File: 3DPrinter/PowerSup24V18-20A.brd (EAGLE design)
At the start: 115 x 161.7 mm, 87 parts, among them IC1 POWER-TNY264PN, T1 TRANS-1/1EFD25-10, T2 _TRANSFORMERS_GDT_20X6.5, T3 TRANS-1/1ETD39, U1 SG3525AN, X1 CON-7.62-02P, X2 CON-7.62-02P

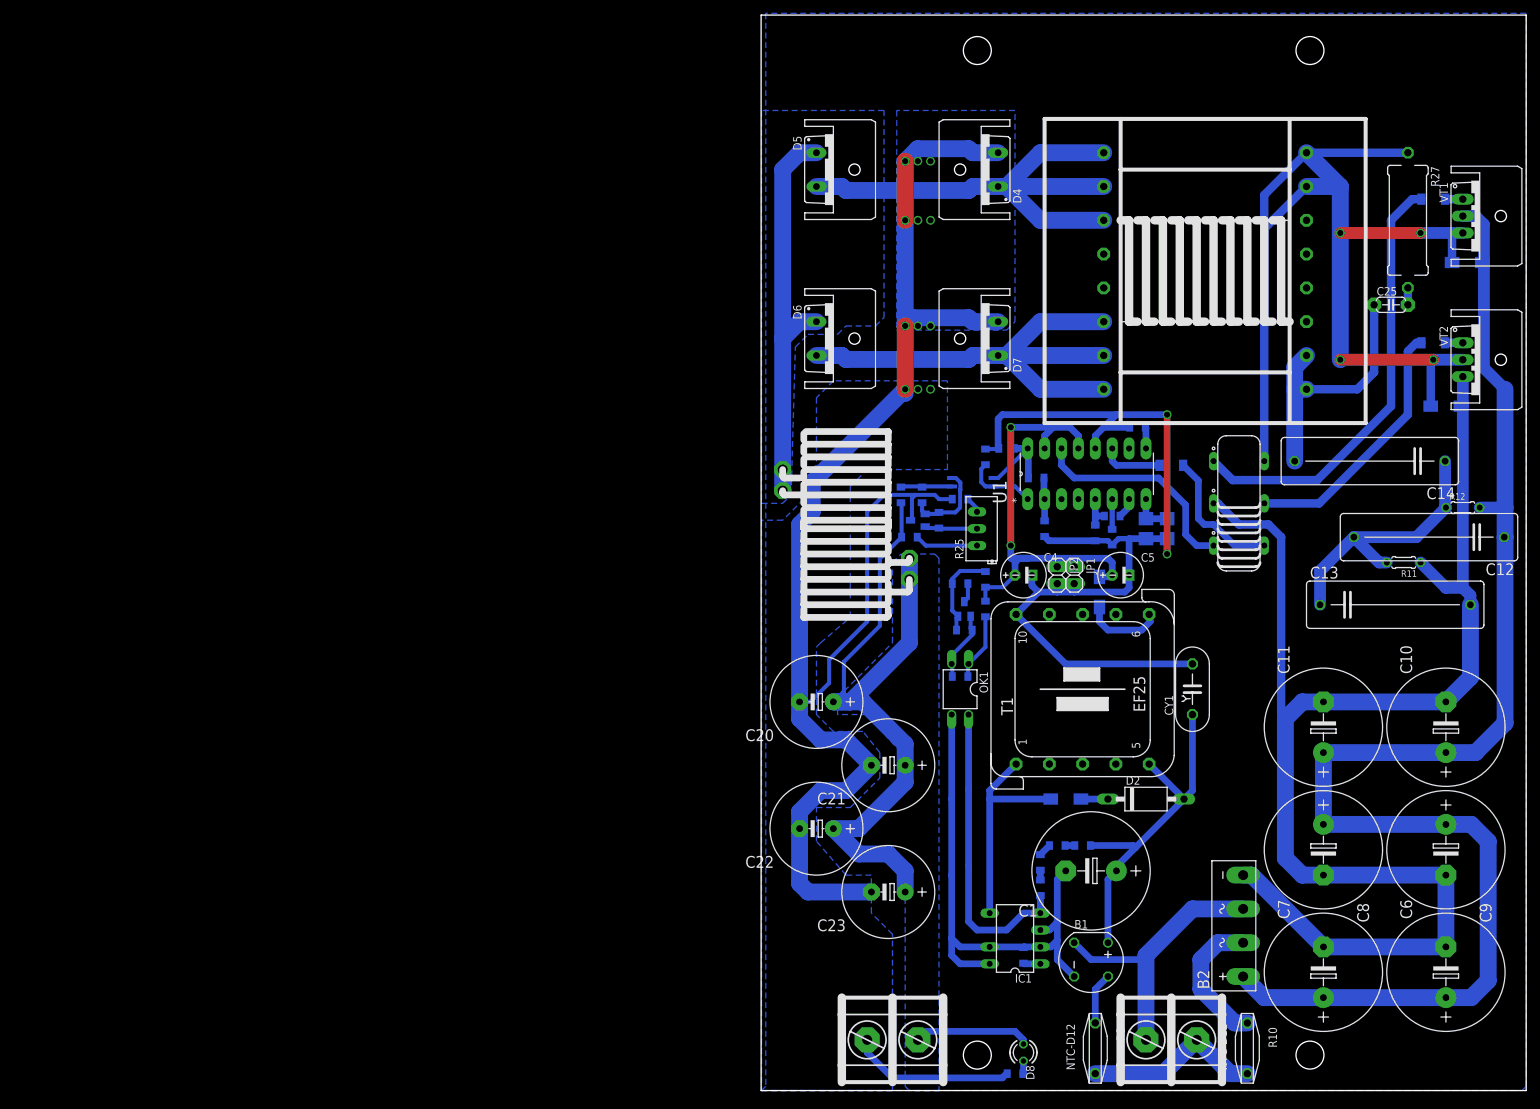
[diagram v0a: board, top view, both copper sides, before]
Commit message: исправил существенные косяки
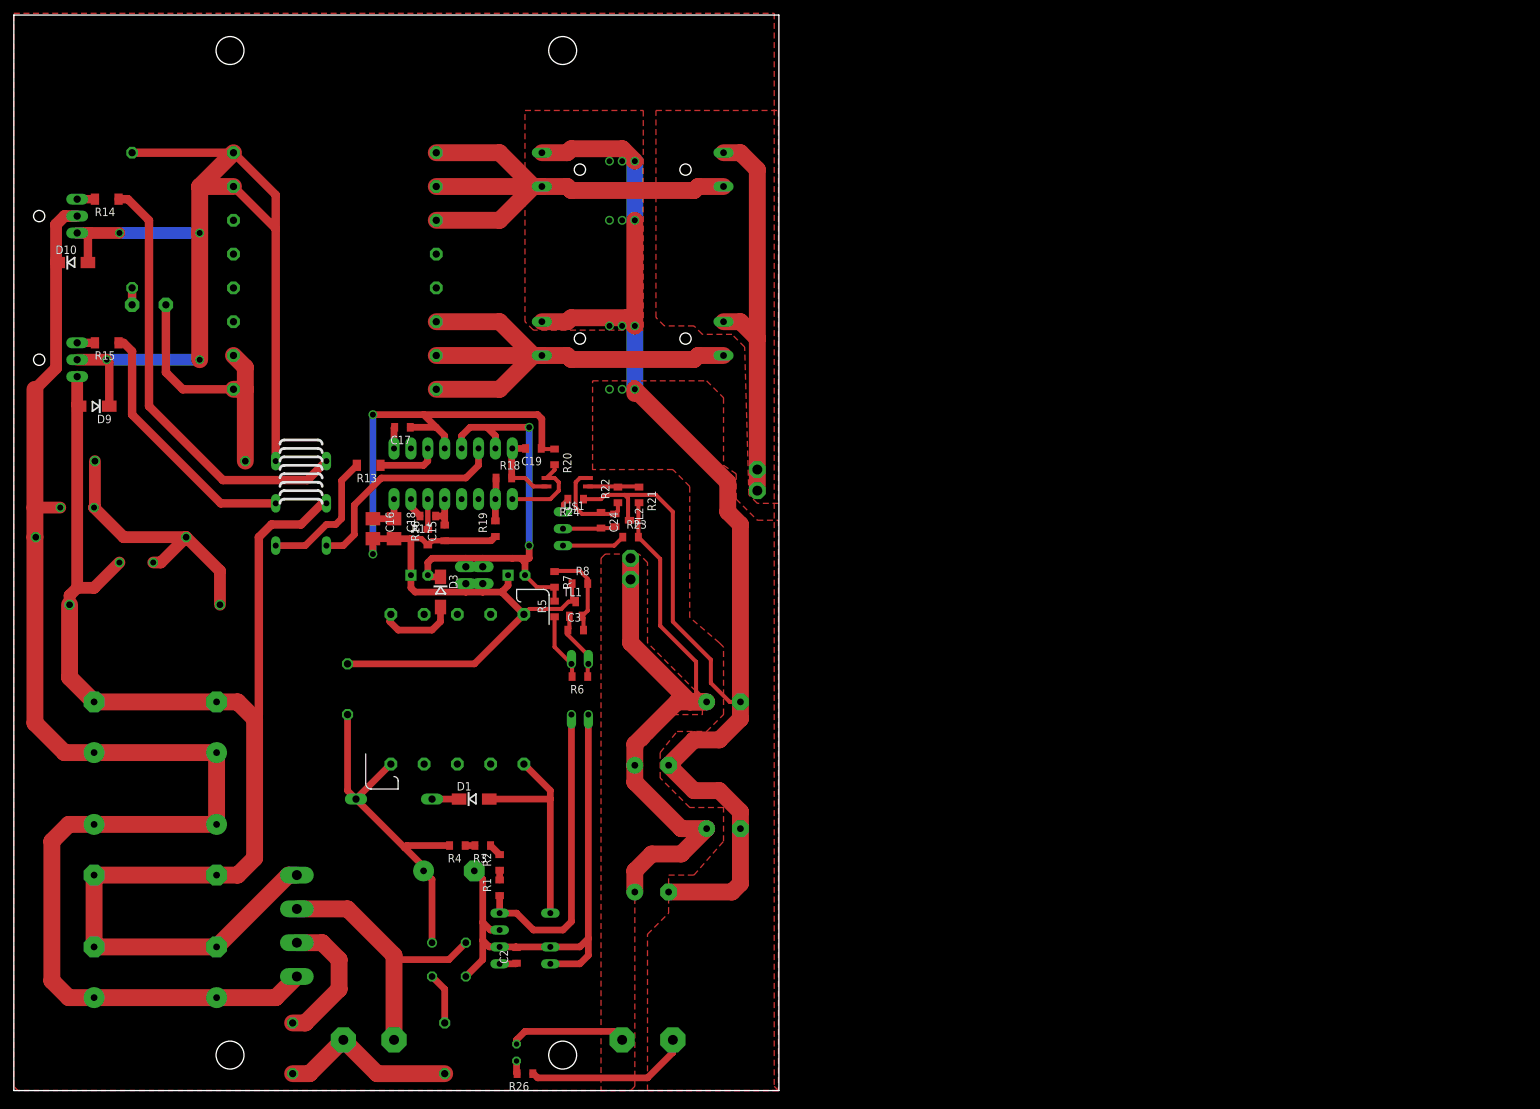
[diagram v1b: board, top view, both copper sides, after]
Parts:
- moved U$2 213.4 mm to (-105.4, 158.1), flipped to the bottom
- moved U$3 213.4 mm to (-105.4, 136.5), flipped to the bottom
- moved VT1 213.4 mm to (-105.4, 158.1), flipped to the bottom
- moved VT2 213.4 mm to (-105.4, 136.5), flipped to the bottom
- moved D10 209.6 mm to (-103.5, 151.1), flipped to the top
- moved R12 208.3 mm to (-102.9, 114.3), flipped to the bottom
- moved C10 203.2 mm to (-100.3, 81.3), flipped to the bottom
- moved C6 203.2 mm to (-100.3, 44.5), flipped to the bottom
- moved C9 203.2 mm to (-100.3, 62.9), flipped to the bottom
- moved D9 203.2 mm to (-100.3, 129.5), flipped to the top
- moved R14 199.4 mm to (-98.4, 160.7), flipped to the top
- moved R15 199.4 mm to (-98.4, 139.1), flipped to the top
- moved C12 198.1 mm to (-97.8, 109.9), flipped to the bottom
- moved R27 191.8 mm to (-94.6, 157.5), flipped to the bottom
- moved R11 190.5 mm to (-94.0, 106.0), flipped to the bottom
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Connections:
- removed net N$17: R8.1, TL1.3
- net GND: now also R8.1, TL1.3
- net N$31: now also U$1.4; no longer U$1.3
- net N$36: now also U$1.3; no longer U$1.4
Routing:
- net GND: track 146.2 -> 157.7 mm
- net N$17: track 2.93 -> 0.00 mm
- net N$36: track 10.9 -> 13.4 mm
- net +12V: track 69.7 -> 68.0 mm
- net FB2: track 12.8 -> 14.4 mm
- net N$31: track 13.5 -> 12.2 mm
- net N$38: track 247.6 -> 248.3 mm
- added copper zone on layer 1, net N$37
- added copper zone on layer 1, net N$38
- added copper zone on layer 1, net N$39
- added copper zone on layer 1, net N$52
- removed copper zone on layer 16, net N$37
- removed copper zone on layer 16, net N$38
- removed copper zone on layer 16, net N$39
- removed copper zone on layer 16, net N$52
